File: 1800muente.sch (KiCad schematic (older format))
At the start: 163 parts, among them K1 MX-1U, K10 MX-1U, K11 MX-1U, K12 MX-1U, K13 MX-1U, K14 MX-1U, K15 MX-1U, K16 MX-1U, K17 MX-1U, K18 MX-1U, K19 MX-1U, K2 MX-1U, K20 MX-1U, K21 MX-1U, K22 MX-1U, K23 MX-1U, K24 MX-1U, K25 MX-1U, K26 MX-1U, K27 MX-1U, K28 MX-1U, K29 MX-1U, K3 MX-1U, K30 MX-1U, K31 MX-1U, K32 MX-1U, K33 MX-1U, K34 MX-1U, K35 MX-1U, K36 MX-1U, K37 MX-1U, K38 MX-1U, K39 MX-1U, K4 MX-1U, K40 MX-1U, K41 MX-1U, K42 MX-1U, K43 MX-1U, K44 MX-1U, K45 MX-1U, K46 MX-1U, K47 MX-1U, K48 MX-1U, K49 MX-1U, K5 MX-1U, K50 MX-1U, K51 MX-1U, K52 MX-1U, K53 MX-1U, K54 MX-1U, K55 MX-1U, K56 MX-1U, K57 MX-1U, K58 MX-1U, K59 MX-1U, K6 MX-1U, K60 MX-1U, K61 MX-1U, K62 MX-1U, K63 MX-1U, K64 MX-1U, K65 MX-1U, K66 MX-1U, K67 MX-1U, K68 MX-1U, K69 MX-1U, K7 MX-1U, K70 MX-1U, K71 MX-1U, K72 MX-1U, K73 MX-1U, K74 MX-1U, K75 MX-1U, K76 MX-1U, K77 MX-1U, K78 MX-1U, K79 MX-1U, K8 MX-1U, K80 MX-1U, K81 MX-1U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

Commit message: aligning switches
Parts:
- K61: footprint MX_Alps_Hybrid:MXOnly-2U-NoLED -> MX_Alps_Hybrid:MXOnly-ISO
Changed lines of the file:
@@
 F 0 "K61" H 11086 6817 60  0000 C CNN
 F 1 "MX-1U" H 11086 6743 20  0000 C CNN
-F 2 "MX_Alps_Hybrid:MXOnly-2U-NoLED" H 10975 6575 60  0001 C CNN
+F 2 "MX_Alps_Hybrid:MXOnly-ISO" H 10975 6575 60  0001 C CNN
 F 3 "" H 10975 6575 60  0001 C CNN
 	1    11000 6600

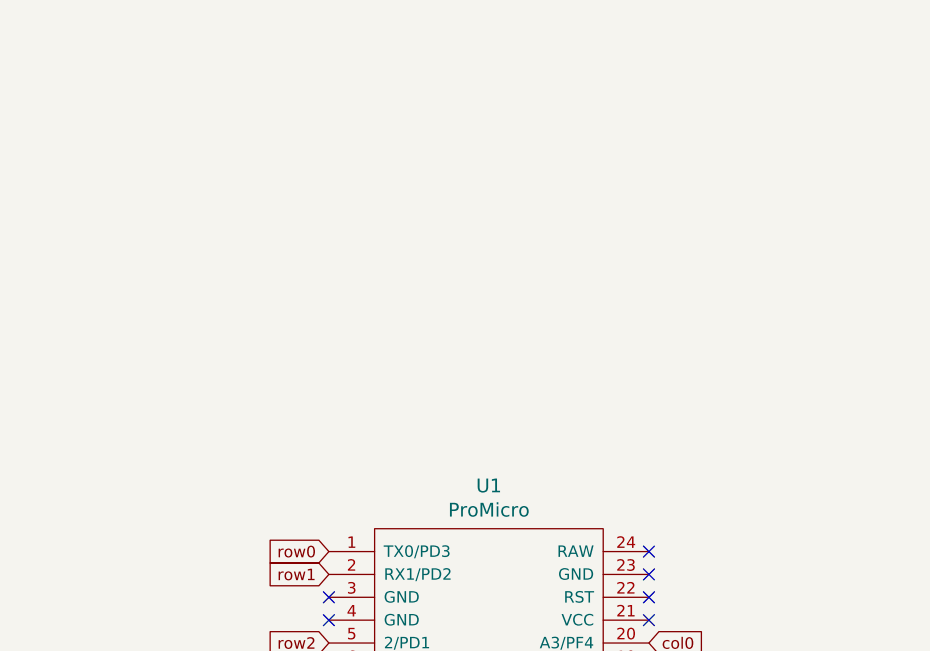
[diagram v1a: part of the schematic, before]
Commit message: brb
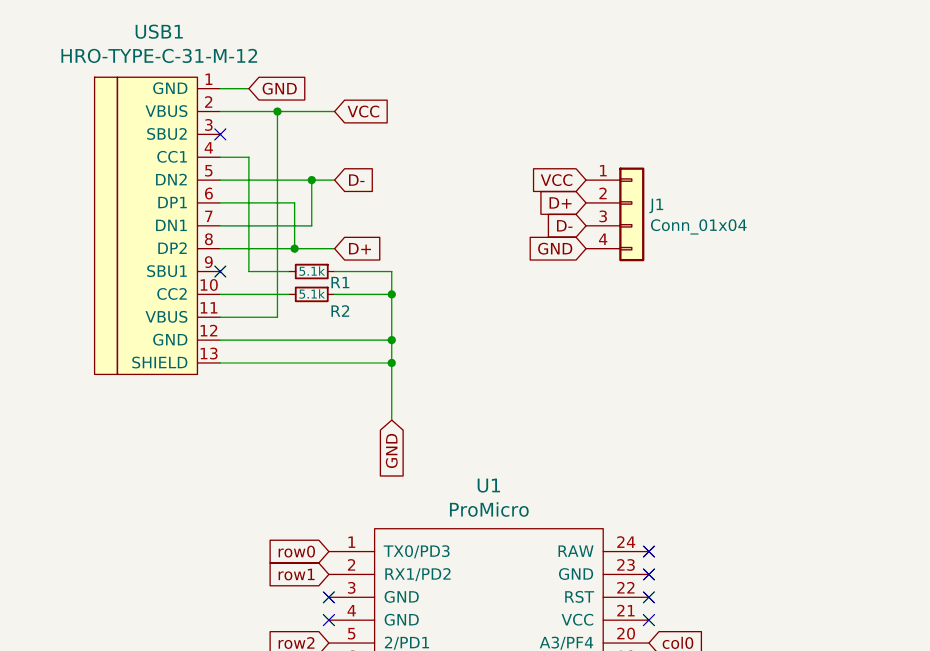
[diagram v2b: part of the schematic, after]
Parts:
- added J1: Conn_01x04, Connector_PinSocket_2.54mm:PinSocket_1x04_P2.54mm_Vertical, symbol Connector_Generic:Conn_01x04
- added R1, R2: 5.1k, Keebio-Parts:Resistor, symbol Device:R_Small
- added USB1: HRO-TYPE-C-31-M-12, Type-C:HRO-TYPE-C-31-M-12-HandSoldering, symbol keebio:HRO-TYPE-C-31-M-12
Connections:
- new net: R1.2, USB1.4 (CC1)
- new net: R2.2, USB1.10 (CC2)
- new net D+: J1.2 (Pin_2), USB1.6 (DP1), USB1.8 (DP2)
- new net D-: J1.3 (Pin_3), USB1.5 (DN2), USB1.7 (DN1)
- new net GND: J1.4 (Pin_4), R1.1, R2.1, USB1.1 (GND), USB1.12 (GND), USB1.13 (SHIELD)
- new net VCC: J1.1 (Pin_1), USB1.11 (VBUS), USB1.2 (VBUS)
- no-connect marks 6 -> 8
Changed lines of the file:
@@
 NoConn ~ 5050 3900
 NoConn ~ 5050 3800
+$Comp
+L keebio:HRO-TYPE-C-31-M-12 USB1
+U 1 1 5CEF2187
+P 3075 2325
+F 0 "USB1" H 2908 3122 60  0000 C CNN
+F 1 "HRO-TYPE-C-31-M-12" H 2908 3016 60  0000 C CNN
+F 2 "Type-C:HRO-TYPE-C-31-M-12-HandSoldering" H 3075 2325 60  0001 C CNN
+F 3 "" H 3075 2325 60  0001 C CNN
+	1    3075 2325
+	1    0    0    -1
+$EndComp
+$Comp
+L Connector_Generic:Conn_01x04 J1
+U 1 1 5CF08108
+P 4975 2275
+F 0 "J1" H 5055 2267 50  0000 L CNN
+F 1 "Conn_01x04" H 5055 2176 50  0000 L CNN
+F 2 "Connector_PinSocket_2.54mm:PinSocket_1x04_P2.54mm_Vertical" H 4975 2275 50  0001 C CNN
+F 3 "~" H 4975 2275 50  0001 C CNN
+	1    4975 2275
+	1    0    0    -1
+$EndComp
+Wire Wire Line
+	3175 2975 3925 2975
+Wire Wire Line
+	3925 2975 3925 3225
+Wire Wire Line
+	3175 2875 3925 2875
+Wire Wire Line
+	3925 2875 3925 2975
+Connection ~ 3925 2975
+Wire Wire Line
+	3925 2675 3925 2875
+Connection ~ 3925 2875
+$Comp
+L Device:R_Small R2
+U 1 1 5CEC0033
+P 3575 2675
+F 0 "R2" V 3650 2800 50  0000 C CNN
+F 1 "5.1k" V 3575 2675 39  0000 C CNN
+F 2 "Keebio-Parts:Resistor" H 3575 2675 50  0001 C CNN
+F 3 "~" H 3575 2675 50  0001 C CNN
+	1    3575 2675
+	0    1    1    0
+$EndComp
+Wire Wire Line
+	3675 2675 3925 2675
+Wire Wire Line
+	3175 2675 3475 2675
+NoConn ~ 3175 2575
+Wire Wire Line
+	3175 2075 3300 2075
+Wire Wire Line
+	3300 2075 3300 2575
+Wire Wire Line
+	3300 2575 3475 2575
+Wire Wire Line
+	3675 2575 3925 2575
+Wire Wire Line
+	3925 2575 3925 2675
+Connection ~ 3925 2675
+Wire Wire Line
+	3300 1775 3175 1775
+Wire Wire Line
+	3175 1875 3425 1875
+Wire Wire Line
+	3425 1875 3425 2775
+Wire Wire Line
+	3425 2775 3175 2775
+Text GLabel 4775 2175 0    50   Input ~ 0
+VCC
+Text GLabel 4775 2275 0    50   Input ~ 0
+D+
+Text GLabel 4775 2375 0    50   Input ~ 0
+D-
+Text GLabel 4775 2475 0    50   Input ~ 0
+GND
+Text GLabel 3300 1775 2    50   Input ~ 0
+GND
+Text GLabel 3925 3225 3    50   Input ~ 0
+GND
+Text GLabel 3675 1875 2    50   Input ~ 0
+VCC
+Wire Wire Line
+	3675 1875 3425 1875
+Connection ~ 3425 1875
+NoConn ~ 3175 1975
+Text GLabel 3675 2175 2    50   Input ~ 0
+D-
+Text GLabel 3675 2475 2    50   Input ~ 0
+D+
+Wire Wire Line
+	3675 2175 3575 2175
+$Comp
+L Device:R_Small R1
+U 1 1 5CEAB997
+P 3575 2575
+F 0 "R1" V 3625 2700 50  0000 C CNN
+F 1 "5.1k" V 3575 2575 39  0000 C CNN
+F 2 "Keebio-Parts:Resistor" H 3575 2575 50  0001 C CNN
+F 3 "~" H 3575 2575 50  0001 C CNN
+	1    3575 2575
+	0    1    1    0
+$EndComp
+Wire Wire Line
+	3175 2475 3500 2475
+Wire Wire Line
+	3175 2275 3500 2275
+Wire Wire Line
+	3500 2275 3500 2475
+Connection ~ 3500 2475
+Wire Wire Line
+	3500 2475 3675 2475
+Wire Wire Line
+	3175 2375 3575 2375
+Wire Wire Line
+	3575 2375 3575 2175
+Connection ~ 3575 2175
+Wire Wire Line
+	3575 2175 3175 2175
 $EndSCHEMATC
